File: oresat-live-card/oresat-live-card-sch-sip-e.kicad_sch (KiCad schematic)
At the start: 1 part, among them U7 OSD3358-512M-BSM

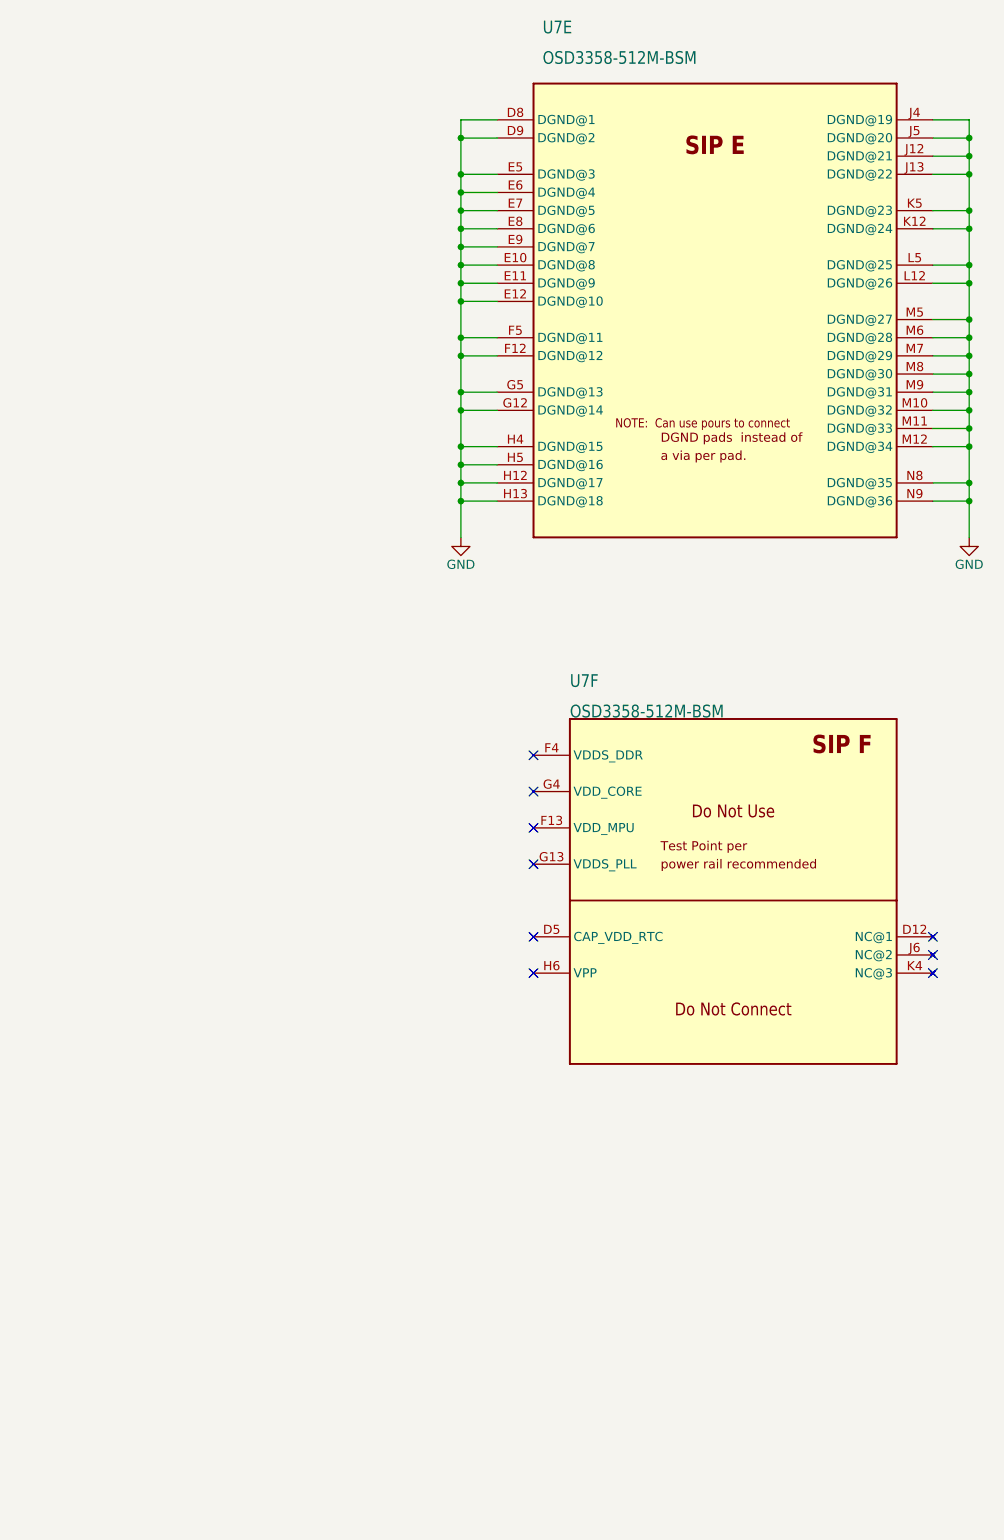
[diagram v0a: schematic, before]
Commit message: mostly just polish after BOM fixes
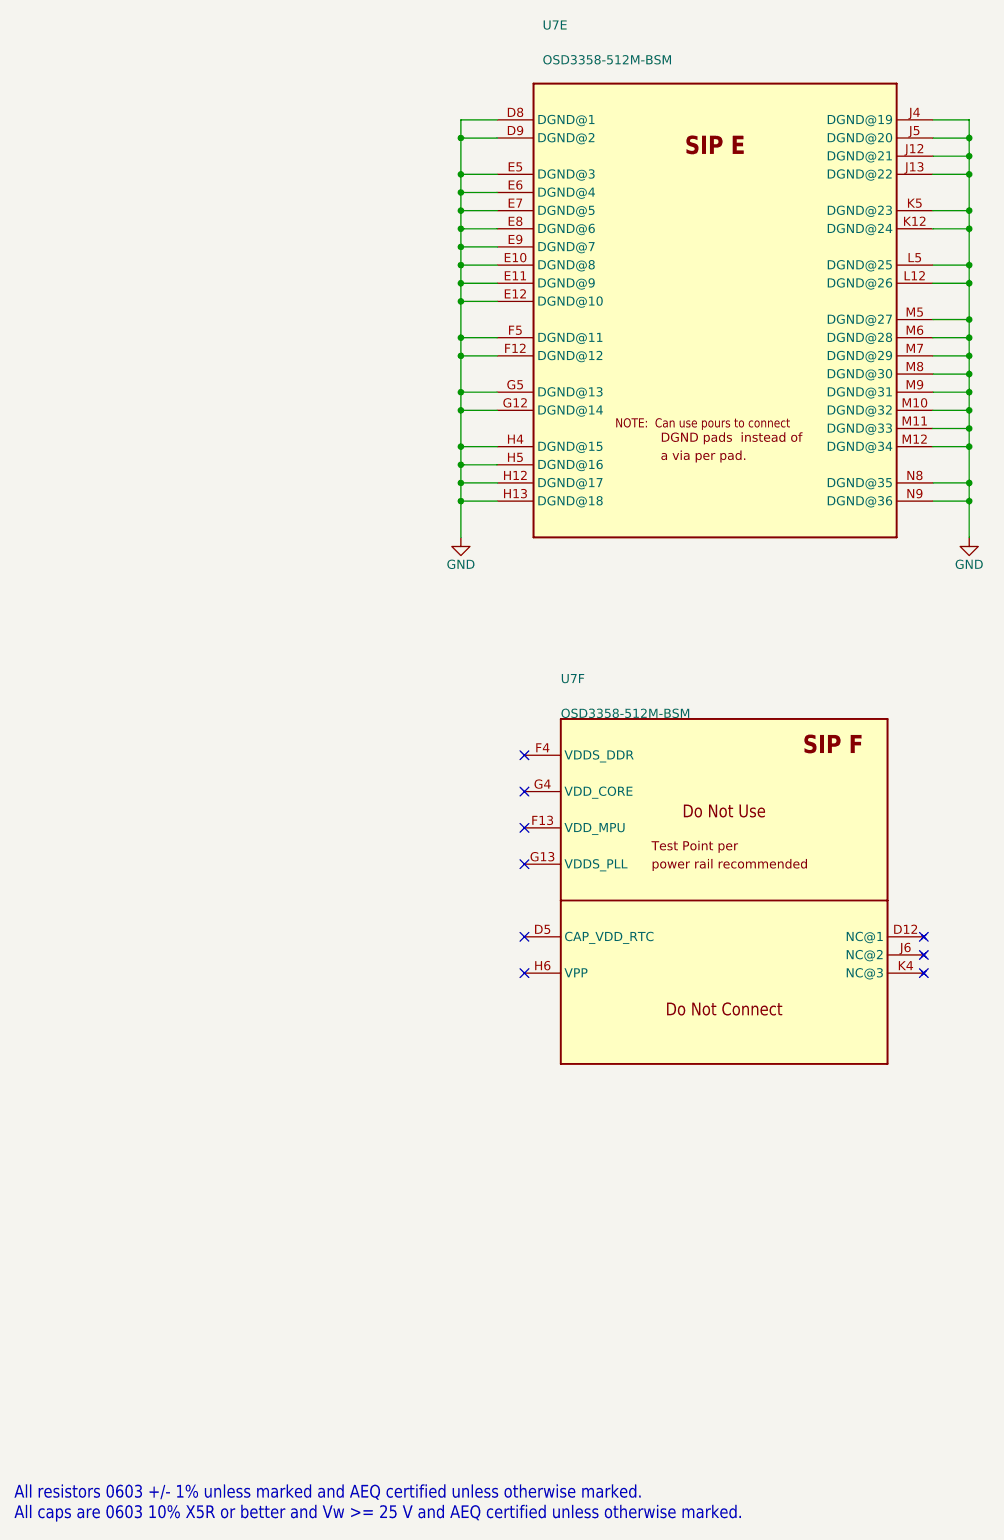
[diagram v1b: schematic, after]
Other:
- note added: "All resistors 0603 +/- 1% unless marked and AEQ certified unless otherwise marked. All caps are 0603 10% X5R or better and Vw >= 25 V and AEQ certified unless otherwise marked."
- moved on the sheet: U7F
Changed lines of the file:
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@@
 		(rev "2.1")
 	)
+	(text "All resistors 0603 +/- 1% unless marked and AEQ certified unless otherwise marked.\nAll caps are 0603 10% X5R or better and Vw >= 25 V and AEQ certified unless otherwise marked."
+		(exclude_from_sim no)
+		(at 114.046 265.938 0)
+		(effects
+			(font
+				(size 1.778 1.5113)
+			)
+			(justify left bottom)
+		)
+	)
 	(junction
 		(at 247.65 100.33)
@@
 	)
 	(no_connect
-		(at 186.69 163.83)
+		(at 185.42 163.83)
 	)
 	(no_connect
-		(at 242.57 189.23)
+		(at 241.3 189.23)
 	)
 	(no_connect
-		(at 242.57 186.69)
+		(at 241.3 186.69)
 	)
 	(no_connect
-		(at 186.69 189.23)
+		(at 185.42 189.23)
 	)
 	(no_connect
-		(at 242.57 184.15)
+		(at 241.3 184.15)
 	)
 	(no_connect
-		(at 186.69 168.91)
+		(at 185.42 168.91)
 	)
 	(no_connect
-		(at 186.69 184.15)
+		(at 185.42 184.15)
 	)
 	(no_connect
-		(at 186.69 173.99)
+		(at 185.42 173.99)
 	)
 	(no_connect
-		(at 186.69 158.75)
+		(at 185.42 158.75)
 	)
 	(wire
@@
 			(effects
 				(font
-					(size 1.778 1.5113)
+					(size 1.27 1.27)
 				)
 				(justify left top)
@@
 			(effects
 				(font
-					(size 1.778 1.5113)
+					(size 1.27 1.27)
 				)
 				(justify left bottom)
@@
 	(symbol
 		(lib_id "oresat-ics:OSD3358-512M-BSM")
-		(at 214.63 179.07 0)
+		(at 213.36 179.07 0)
 		(unit 6)
 		(body_style 1)
@@
 		(dnp no)
 		(property "Reference" "U7"
-			(at 191.77 147.32 0)
-			(show_name no)
-			(do_not_autoplace no)
-			(effects
-				(font
-					(size 1.778 1.5113)
+			(at 190.5 147.32 0)
+			(show_name no)
+			(do_not_autoplace no)
+			(effects
+				(font
+					(size 1.27 1.27)
 				)
 				(justify left top)
@@
 		)
 		(property "Value" "OSD3358-512M-BSM"
-			(at 191.77 153.67 0)
-			(show_name no)
-			(do_not_autoplace no)
-			(effects
-				(font
-					(size 1.778 1.5113)
+			(at 190.5 153.67 0)
+			(show_name no)
+			(do_not_autoplace no)
+			(effects
+				(font
+					(size 1.27 1.27)
 				)
 				(justify left bottom)
@@
 		)
 		(property "Footprint" "oresat-ics:U-Octavo-OSD335X-BGA-256"
-			(at 214.63 71.12 0)
+			(at 213.36 71.12 0)
 			(hide yes)
 			(show_name no)
@@
 		)
 		(property "Datasheet" "https://www.ti.com/lit/ds/symlink/tps2041b-q1.pdf?HQS=dis-dk-null-digikeymode-dsf-pf-null-wwe&ts=1651525711603&ref_url=https%253A%252F%252Fwww.ti.com%252Fgeneral%252Fdocs%252Fsuppproductinfo.tsp%253FdistId%253D10%2526gotoUrl%253Dhttps%253A%252F%252Fwww.ti.com%252Flit%252Fgpn%252Ftps2041b-q1"
-			(at 214.63 179.07 0)
+			(at 213.36 179.07 0)
 			(hide yes)
 			(show_name no)
@@
 		)
 		(property "Description" "OSD335x Embedded Module 1GHz 512MB"
-			(at 214.63 179.07 0)
+			(at 213.36 179.07 0)
 			(hide yes)
 			(show_name no)
@@
 		)
 		(property "MPN" "OSD3358-512M-BSM"
-			(at 214.63 179.07 0)
+			(at 213.36 179.07 0)
 			(hide yes)
 			(show_name no)
@@
 		)
 		(property "DPN" "1676-1002-ND"
-			(at 214.63 179.07 0)
+			(at 213.36 179.07 0)
 			(hide yes)
 			(show_name no)
@@
 		)
 		(property "MFR" "Octavo Systems"
-			(at 214.63 179.07 0)
+			(at 213.36 179.07 0)
 			(hide yes)
 			(show_name no)
@@
 		)
 		(property "DIS" "DigiKey"
-			(at 214.63 179.07 0)
-			(hide yes)
-			(show_name no)
+			(at 213.36 179.07 0)
+			(hide yes)
+			(show_name no)
